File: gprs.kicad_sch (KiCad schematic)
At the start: 8 parts, among them J3 Conn_Coaxial, J4 SIM_Card

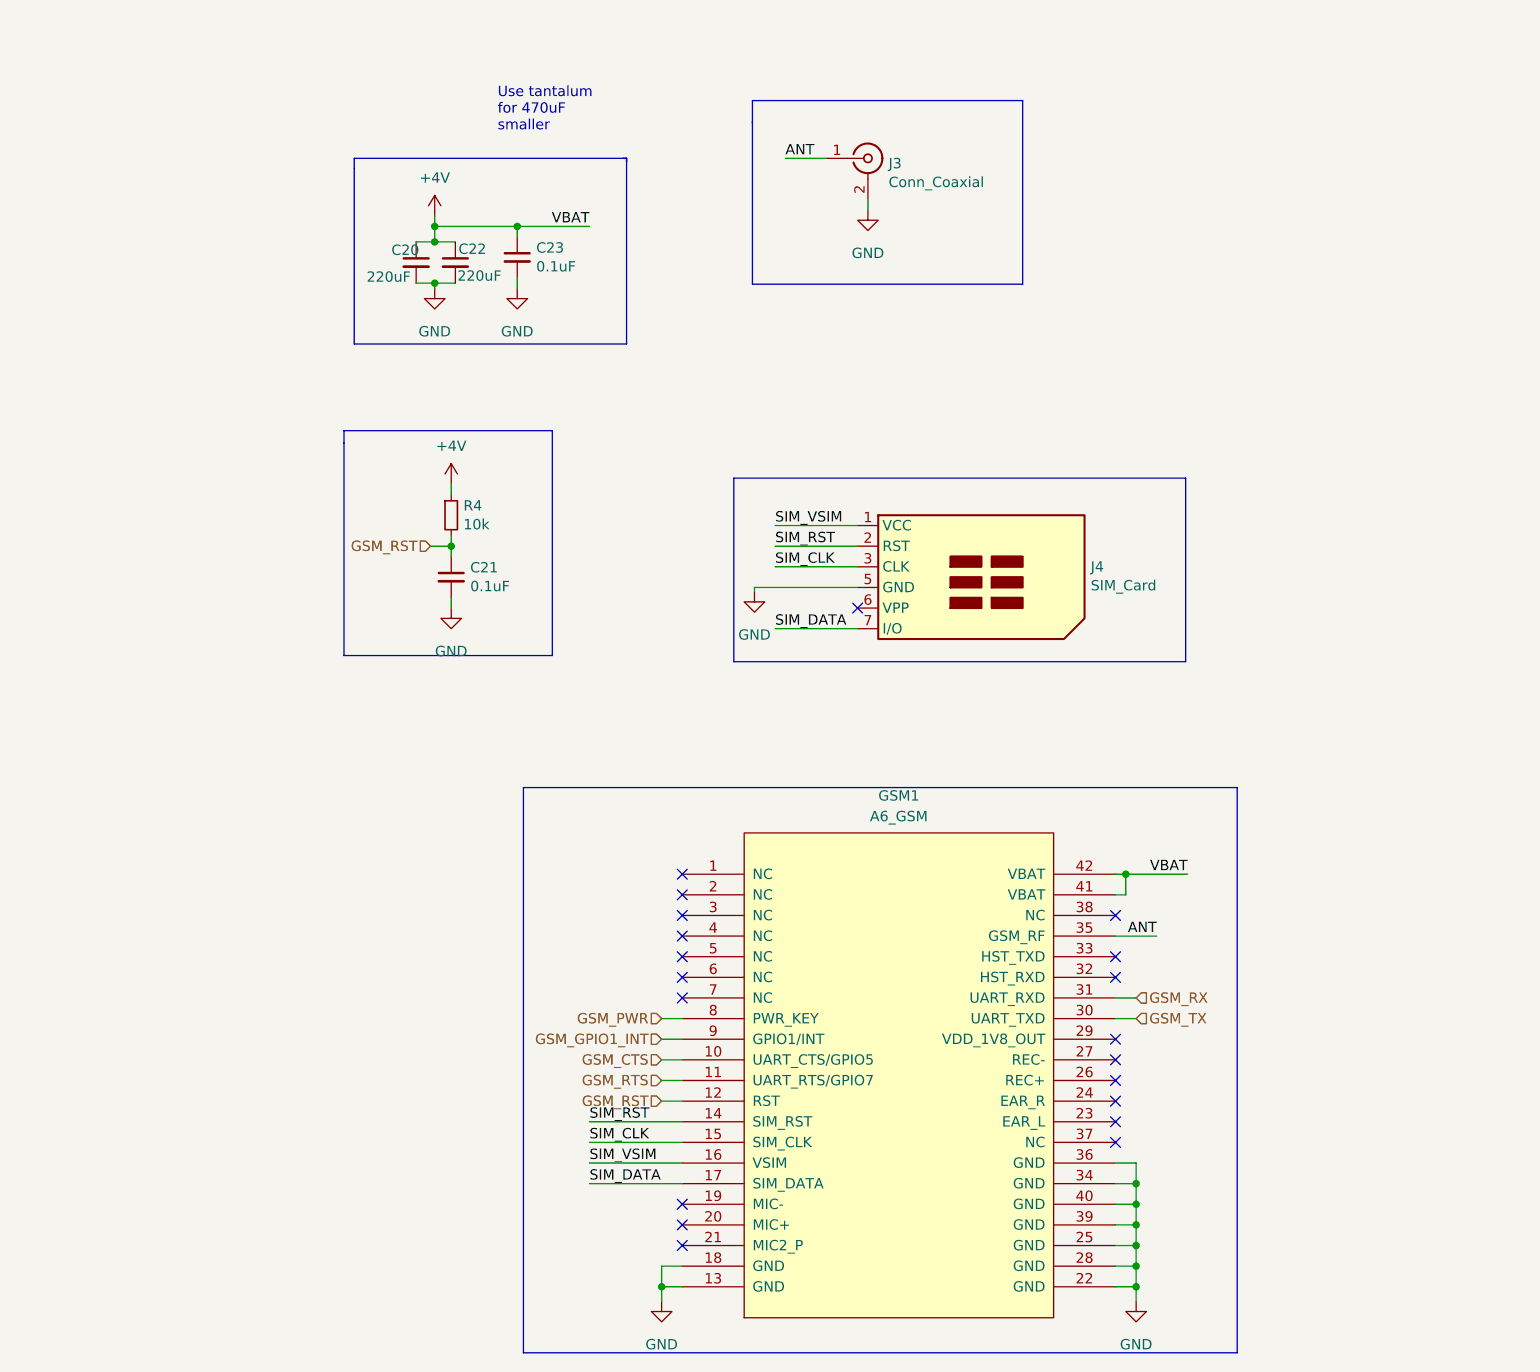
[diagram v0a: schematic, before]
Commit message: KiCad 0.3v
Improved aesthetics.
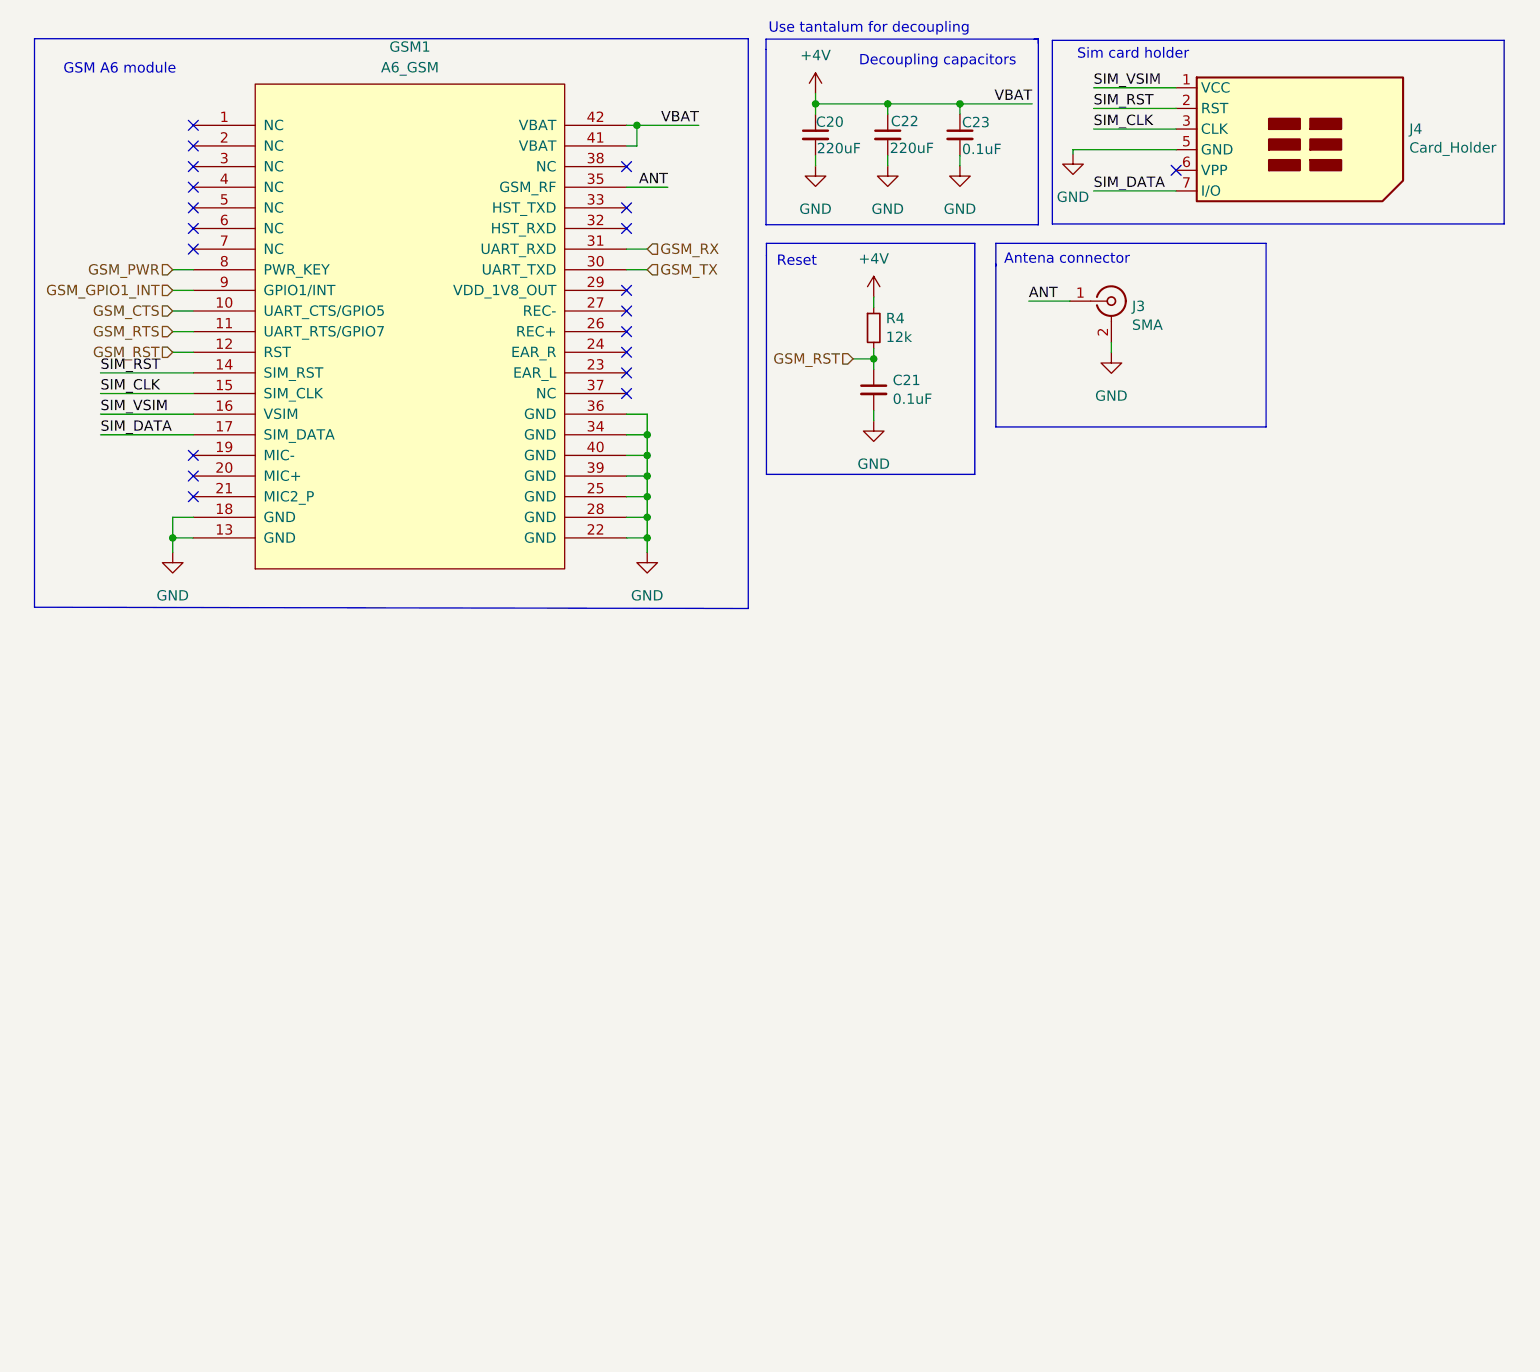
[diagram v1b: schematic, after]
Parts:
- GSM1: symbol test:A6_GSM -> schematics:A6_GSM
- J3: value Conn_Coaxial -> SMA
- J4: value SIM_Card -> Card_Holder
- R4: value 10k -> 12k
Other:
- note added: "Antena connector"
- note added: "Decoupling capacitors"
- note added: "GSM A6 module"
- note added: "Reset"
- note added: "Sim card holder"
- note added: "Use tantalum for decoupling"
- note removed: "Use tantalum for 470uF smaller"
- moved on the sheet: C21, C22, C23, GSM1, J3, J4, R4
